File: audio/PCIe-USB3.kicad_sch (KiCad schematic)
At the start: 54 parts, among them J3 USB3_A, Q1 DMG1012T, U2 AP3429KTTR-G1, U3 VL805, U4 AP22653W6, Y1 25MHz

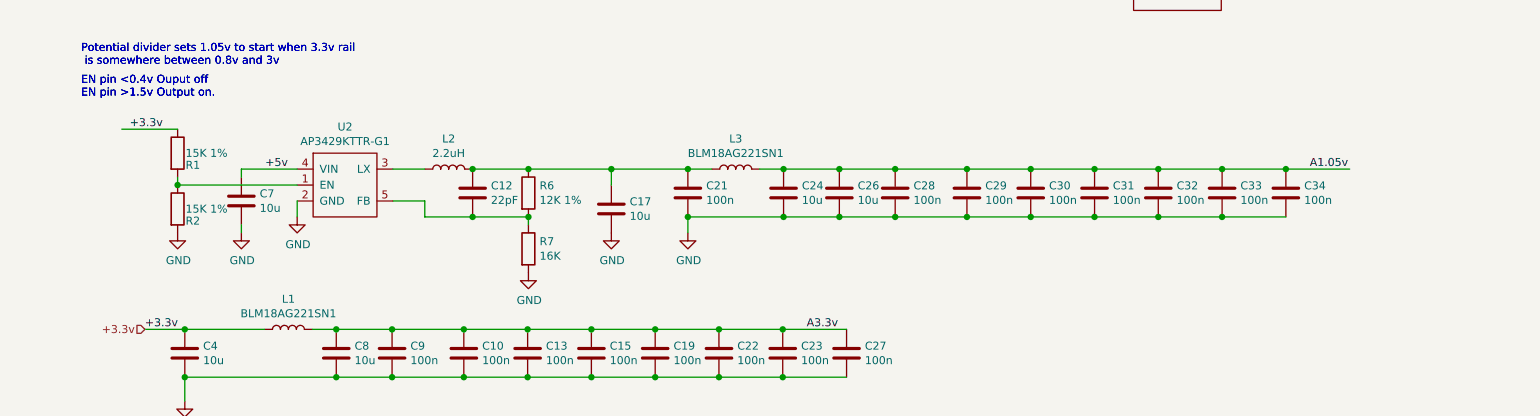
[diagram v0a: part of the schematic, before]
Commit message: .
.
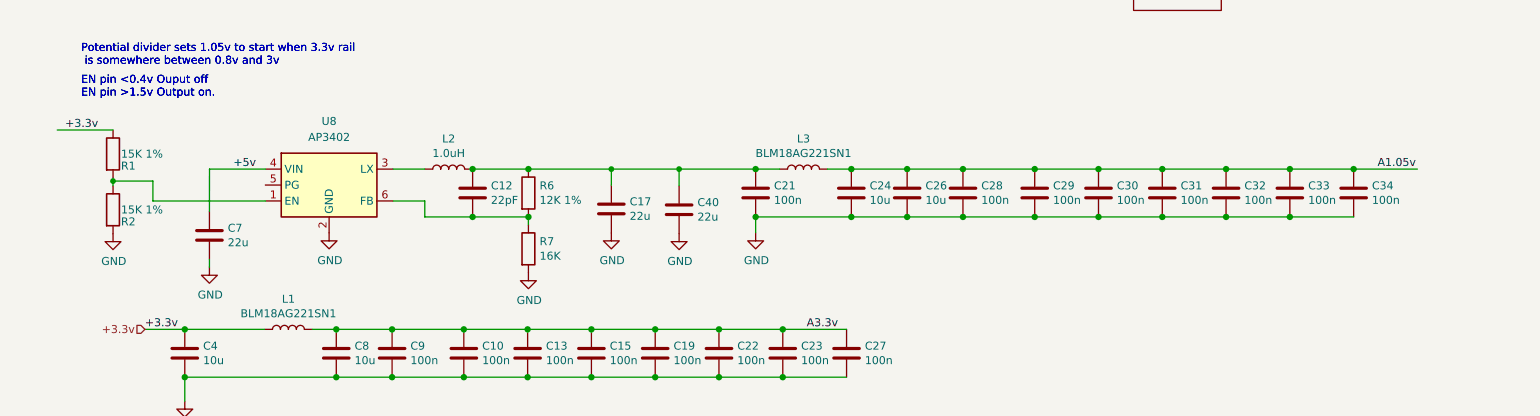
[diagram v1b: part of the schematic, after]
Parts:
- removed U2: AP3429KTTR-G1, Package_TO_SOT_SMD:TSOT-23-5, symbol CM4:AP3429KTTR-G1
- added C40: 22u, Capacitor_SMD:C_0805_2012Metric, symbol Device:C
- added U8: AP3402, Package_TO_SOT_SMD:TSOT-23-6, symbol Regulator_Switching:AP3402
- C17, C7: value 10u -> 22u
- L2: value 2.2uH -> 1.0uH
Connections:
- net +5v: now also U8.4 (VIN)
- net GND: now also C40.2, U8.2 (GND)
- net at C12.1, C17.1, C21.1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: now also C40.1
- net at C12.2, R6.2, R7.1: now also U8.6 (FB)
- net at R1.2, R2.1: now also U8.1 (EN)
- net at L2.1: now also U8.3 (LX)
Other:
- moved on the sheet: C21, C24, C26, C28, C29, C30, C31, C32, C33, C34, C7, L3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
